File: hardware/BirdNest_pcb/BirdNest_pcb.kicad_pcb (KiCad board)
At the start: 2 copper layers, 94 x 78.2 mm, 33 parts, among them J1 Solarpanel, J2 AM312 connector, Q1 FQP27P06, Q5 FQP27P06, U1 DS18B20, U4 ESP32-CAM, U5 TP4056_Module, U6 VXO7803-500

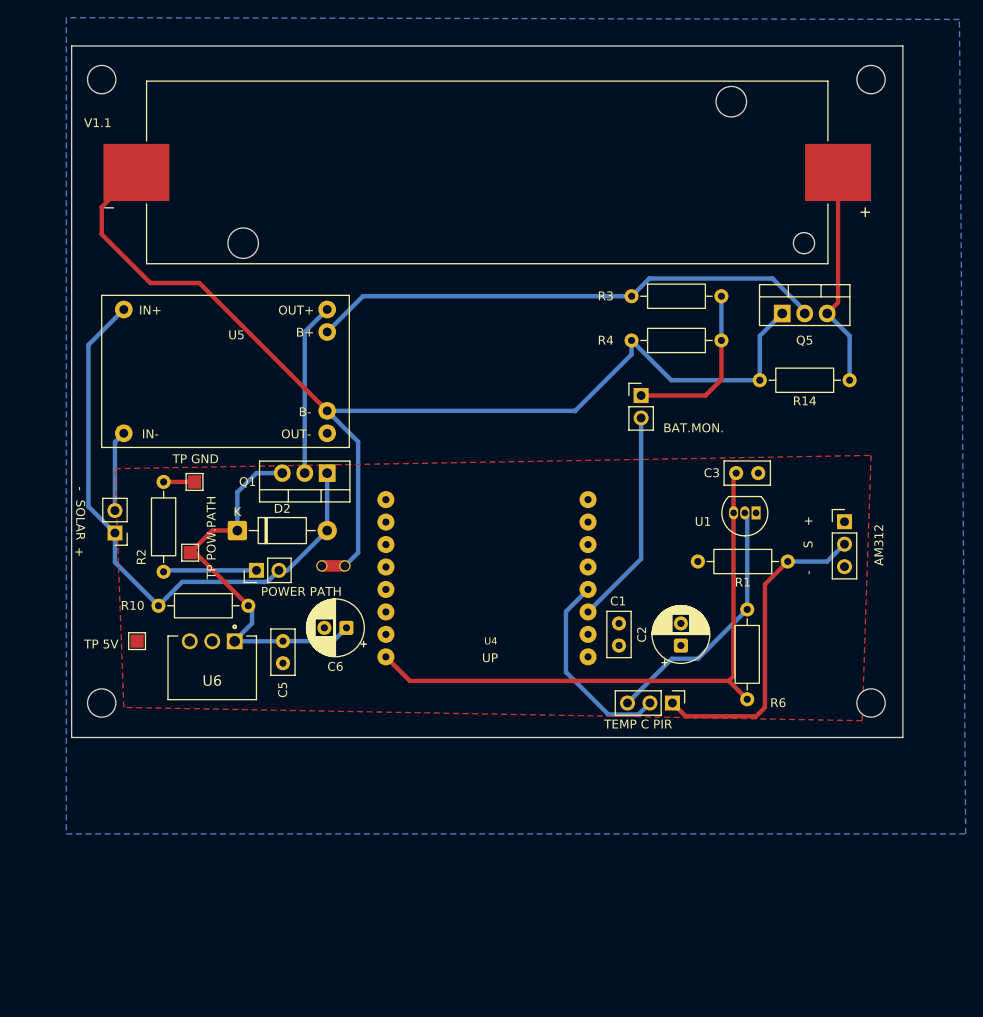
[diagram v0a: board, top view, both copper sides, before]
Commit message: hw: update BirdNest PCB design files
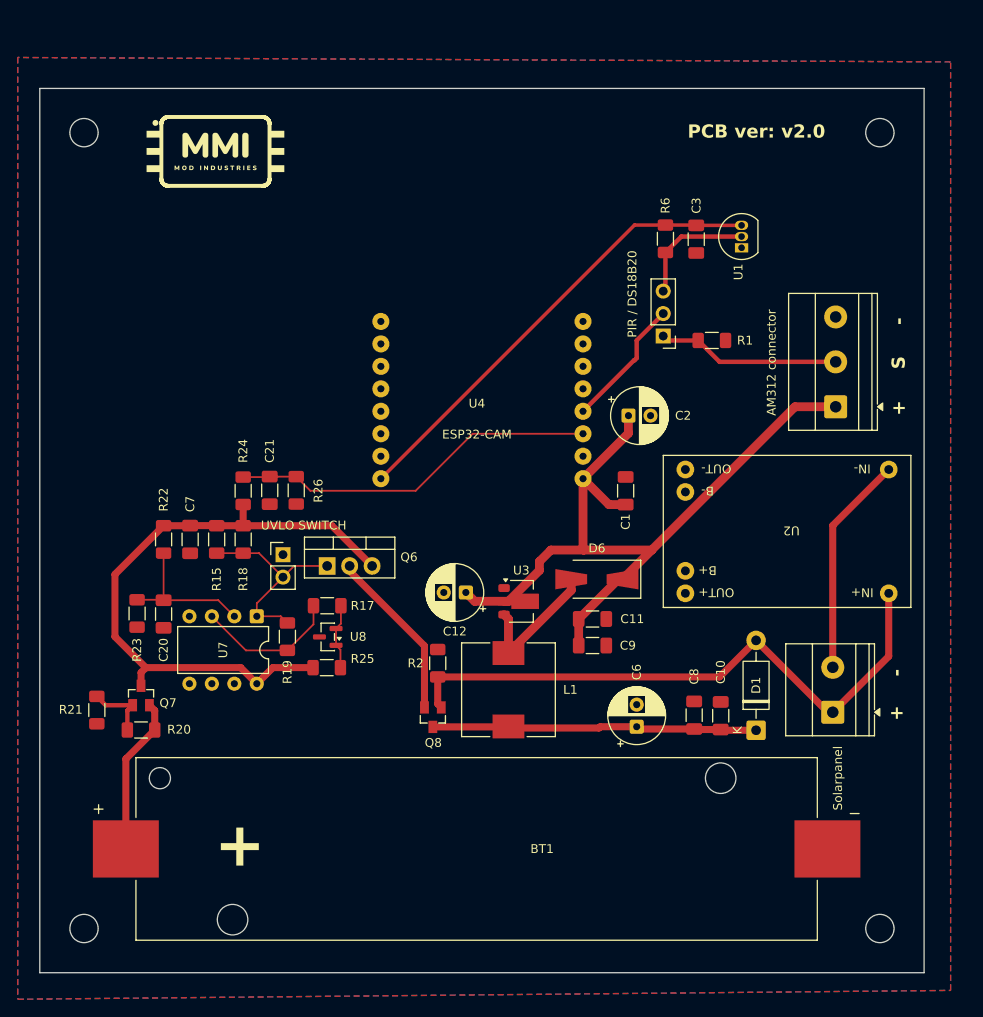
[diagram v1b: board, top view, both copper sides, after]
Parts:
- removed C5: 100nF, Capacitor_THT:C_Disc_D5.0mm_W2.5mm_P2.50mm
- removed D2: 1N5819, Diode_THT:D_DO-41_SOD81_P10.16mm_Horizontal
- removed J1: Solarpanel, Connector_PinHeader_2.54mm:PinHeader_1x02_P2.54mm_Vertical
- removed JP1, JP2: Jumper_2_Open, Connector_PinHeader_2.54mm:PinHeader_1x02_P2.54mm_Vertical
- removed NT2: NetTie_2, NetTie:NetTie-2_THT_Pad1.0mm
- removed Q1, Q5: FQP27P06, Package_TO_SOT_THT:TO-220-3_Vertical
- removed R10: 100k, Resistor_THT:R_Axial_DIN0207_L6.3mm_D2.5mm_P10.16mm_Horizontal
- removed R14: 10k, Resistor_THT:R_Axial_DIN0207_L6.3mm_D2.5mm_P10.16mm_Horizontal
- removed R3: 1,5M, Resistor_THT:R_Axial_DIN0207_L6.3mm_D2.5mm_P10.16mm_Horizontal
- removed R4: 1M, Resistor_THT:R_Axial_DIN0207_L6.3mm_D2.5mm_P10.16mm_Horizontal
- removed TP1, TP2, TP3: TestPoint, TestPoint:TestPoint_Pad_1.5x1.5mm
- removed U5: TP4056_Module, MyFootprints:TP4056-Module
- removed U6: VXO7803-500, VXO7803-500:CONV_VXO7803-500
- added C10: 100nF, Capacitor_SMD:C_1206_3216Metric_Pad1.33x1.80mm_HandSolder, F.Cu at (177.0, 110.9)
- added C11: 100nF, Capacitor_SMD:C_1206_3216Metric_Pad1.33x1.80mm_HandSolder, F.Cu at (162.5, 100.0)
- added C12: 100uF, Capacitor_THT:CP_Radial_D6.3mm_P2.50mm, F.Cu at (148.2, 97.0)
- added C20: 100nF, Capacitor_SMD:C_1206_3216Metric_Pad1.33x1.80mm_HandSolder, F.Cu at (114.0, 99.4)
- added C21: 100nF, Capacitor_SMD:C_1206_3216Metric_Pad1.33x1.80mm_HandSolder, F.Cu at (126.0, 85.5)
- added C7: 100nF, Capacitor_SMD:C_1206_3216Metric_Pad1.33x1.80mm_HandSolder, F.Cu at (117.0, 91.0)
- added C8: 22uF, Capacitor_SMD:C_1206_3216Metric_Pad1.33x1.80mm_HandSolder, F.Cu at (174.0, 110.9)
- added C9: 47uF, Capacitor_SMD:C_1206_3216Metric_Pad1.33x1.80mm_HandSolder, F.Cu at (162.5, 103.0)
- added D1: 1N5819, Diode_THT:D_DO-41_SOD81_P10.16mm_Horizontal, F.Cu at (181.0, 112.6)
- added D6: SS14, Diode_SMD:D_SMA-SMB_Universal_Handsoldering, F.Cu at (163.0, 95.5)
- added J3: Solarpanel, TerminalBlock_Phoenix:TerminalBlock_Phoenix_MKDS-1,5-2-5.08_1x02_P5.08mm_Horizontal, F.Cu at (189.7, 110.5)
- added JP7: Jumper_2_Open, Connector_PinHeader_2.54mm:PinHeader_1x02_P2.54mm_Vertical, F.Cu at (127.5, 92.7)
- added L1: 22uH, Inductor_SMD:L_10.4x10.4_H4.8, F.Cu at (153.0, 108.0)
- added Q6: FQP27P06, Package_TO_SOT_THT:TO-220-3_Vertical, F.Cu at (132.5, 94.0)
- added Q7: DMG2305UX, DMG2305UX:SOT23, F.Cu at (111.5, 108.7)
- added Q8: DMG2305UX, DMG2305UX:SOT23, F.Cu at (144.4, 111.1)
- added R15: 100k, Resistor_SMD:R_1206_3216Metric_Pad1.30x1.75mm_HandSolder, F.Cu at (120.0, 91.0)
- added R17: 22k, Resistor_SMD:R_1206_3216Metric_Pad1.30x1.75mm_HandSolder, F.Cu at (132.5, 98.5)
- added R18: 100k, Resistor_SMD:R_1206_3216Metric_Pad1.30x1.75mm_HandSolder, F.Cu at (123.0, 91.0)
- added R19: 1M, Resistor_SMD:R_1206_3216Metric_Pad1.30x1.75mm_HandSolder, F.Cu at (128.0, 102.0)
- added R20: 1M, Resistor_SMD:R_1206_3216Metric_Pad1.30x1.75mm_HandSolder, F.Cu at (111.5, 112.5)
- added R21: 100k, Resistor_SMD:R_1206_3216Metric_Pad1.30x1.75mm_HandSolder, F.Cu at (106.5, 110.3)
- added R22: 39k, Resistor_SMD:R_1206_3216Metric_Pad1.30x1.75mm_HandSolder, F.Cu at (114.0, 91.0)
- added R23: 100k, Resistor_SMD:R_1206_3216Metric_Pad1.30x1.75mm_HandSolder, F.Cu at (111.0, 99.4)
- added R24: 2M, Resistor_SMD:R_1206_3216Metric_Pad1.30x1.75mm_HandSolder, F.Cu at (123.0, 85.5)
- added R25: 680R, Resistor_SMD:R_1206_3216Metric_Pad1.30x1.75mm_HandSolder, F.Cu at (132.4, 105.5)
- added R26: 1M, Resistor_SMD:R_1206_3216Metric_Pad1.30x1.75mm_HandSolder, F.Cu at (129.0, 85.5)
- added U2: TP4056_Module, MyFootprints:TP4056-Module, F.Cu at (198.5, 81.5)
- added U3: ME2188, Package_TO_SOT_SMD:SOT-89-3, F.Cu at (154.4, 98.0)
- added U7: LM393, Package_DIP:DIP-8_W7.62mm, F.Cu at (124.5, 99.7)
- added U8: TL431DBZ, Package_TO_SOT_SMD:SOT-23, F.Cu at (132.6, 102.0)
- C1, C3: footprint Capacitor_THT:C_Disc_D5.0mm_W2.5mm_P2.50mm -> Capacitor_SMD:C_1206_3216Metric_Pad1.33x1.80mm_HandSolder
- J2: footprint Connector_PinHeader_2.54mm:PinHeader_1x03_P2.54mm_Vertical -> TerminalBlock_Phoenix:TerminalBlock_Phoenix_MKDS-1,5-3-5.08_1x03_P5.08mm_Horizontal
- JP3: value PIR OR DS18B20 -> PIR / DS18B20
- R1, R6: footprint Resistor_THT:R_Axial_DIN0207_L6.3mm_D2.5mm_P10.16mm_Horizontal -> Resistor_SMD:R_1206_3216Metric_Pad1.30x1.75mm_HandSolder
- R2: value 10k -> 100k; footprint Resistor_THT:R_Axial_DIN0207_L6.3mm_D2.5mm_P10.16mm_Horizontal -> Resistor_SMD:R_1206_3216Metric_Pad1.30x1.75mm_HandSolder
- moved H4 109.9 mm to (105.0, 45.0)
- moved H1 96.0 mm to (105.0, 135.0)
- moved H2 91.6 mm to (195.0, 135.0)
- moved BT1 76.5 mm to (149.4, 126.0), turned to 180 degrees
- moved R6 42.9 mm to (170.8, 57.0), turned to 90 degrees
- moved JP3 41.5 mm to (170.5, 68.0), turned to 180 degrees
- moved R2 37.2 mm to (145.0, 105.0), turned to 90 degrees
- moved C6 34.7 mm to (167.5, 112.2), turned to 90 degrees
- moved U1 30.0 mm to (179.4, 58.0), turned to 90 degrees
- moved C3 27.4 mm to (174.2, 57.0), turned to 90 degrees
- moved C2 26.7 mm to (166.6, 77.0), turned to 0 degrees
- moved R1 26.4 mm to (176.0, 68.5), turned to 0 degrees
- moved U4 20.2 mm to (150.0, 60.0)
- moved C1 17.5 mm to (166.2, 85.5)
- moved J2 13.0 mm to (190.0, 76.0), turned to 90 degrees
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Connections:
- BT1 pad N: -BATT -> GND
- C6 pad 1: Net-(D2-K) -> /SYS_PWR
- R2 pad 1: GND -> Net-(D1-A)
- R2 pad 2: Net-(JP2-A) -> GND
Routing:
- net -BATT: track 125.6 -> 0.00 mm
- net /+5V: track 0.03 -> 89.8 mm
- net /BAT_RAW: track 0.00 -> 70.3 mm
- net Net-(D1-A): track 0.00 -> 70.1 mm
- net Net-(D2-A): track 67.5 -> 0.00 mm
- net +BATT: track 58.3 -> 0.00 mm
- net Net-(D2-K): track 44.0 -> 0.00 mm
- net /SYS_PWR: track 0.00 -> 36.9 mm
- net Net-(J3-Pin_2): track 0.00 -> 25.0 mm
- net /UVLO_GATE: track 0.00 -> 23.9 mm
- net Net-(Q1-D): track 19.6 -> 0.00 mm
- net /SYS_BATT_SW: track 0.00 -> 19.5 mm
- net Net-(JP1-A): track 19.2 -> 0.00 mm
- net /BAT_MON: track 24.4 -> 41.8 mm
- net /UVLO_SENSE: track 0.00 -> 17.1 mm
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- added copper zone on F.Cu, net GND
- removed copper zone on F.Cu, net /+5V
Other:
- board size 94 x 78.2 mm -> 100 x 100 mm
- board text added: "PCB ver: v2.0"
- board text added: "UVLO SWITCH"
- board text removed: "AM312"
- board text removed: "BAT.MON."
- board text removed: "POWER PATH"
- board text removed: "SOLAR"
- board text removed: "TEMP C PIR"
- board text removed: "TP 5V"
- board text removed: "TP GND"
- board text removed: "TP POW.PATH"
- board text removed: "UP"
- board text removed: "V1.1"
